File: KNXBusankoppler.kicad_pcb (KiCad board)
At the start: 2 copper layers, 42.2 x 37.3 mm, 6 parts, among them J1 Conn_01x10_Male, J2 Conn_01x04_Male, U1 ProMicro

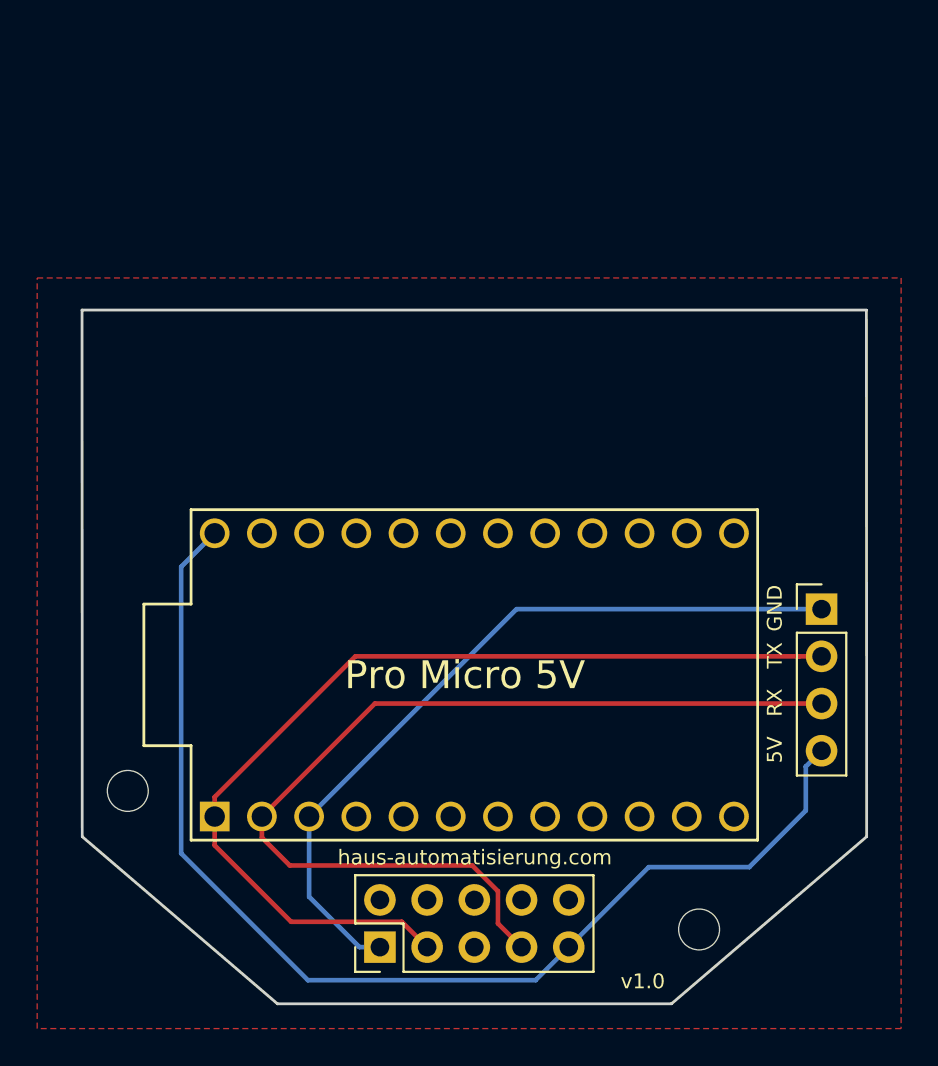
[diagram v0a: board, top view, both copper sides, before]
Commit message: CO2-Sensor 1.0
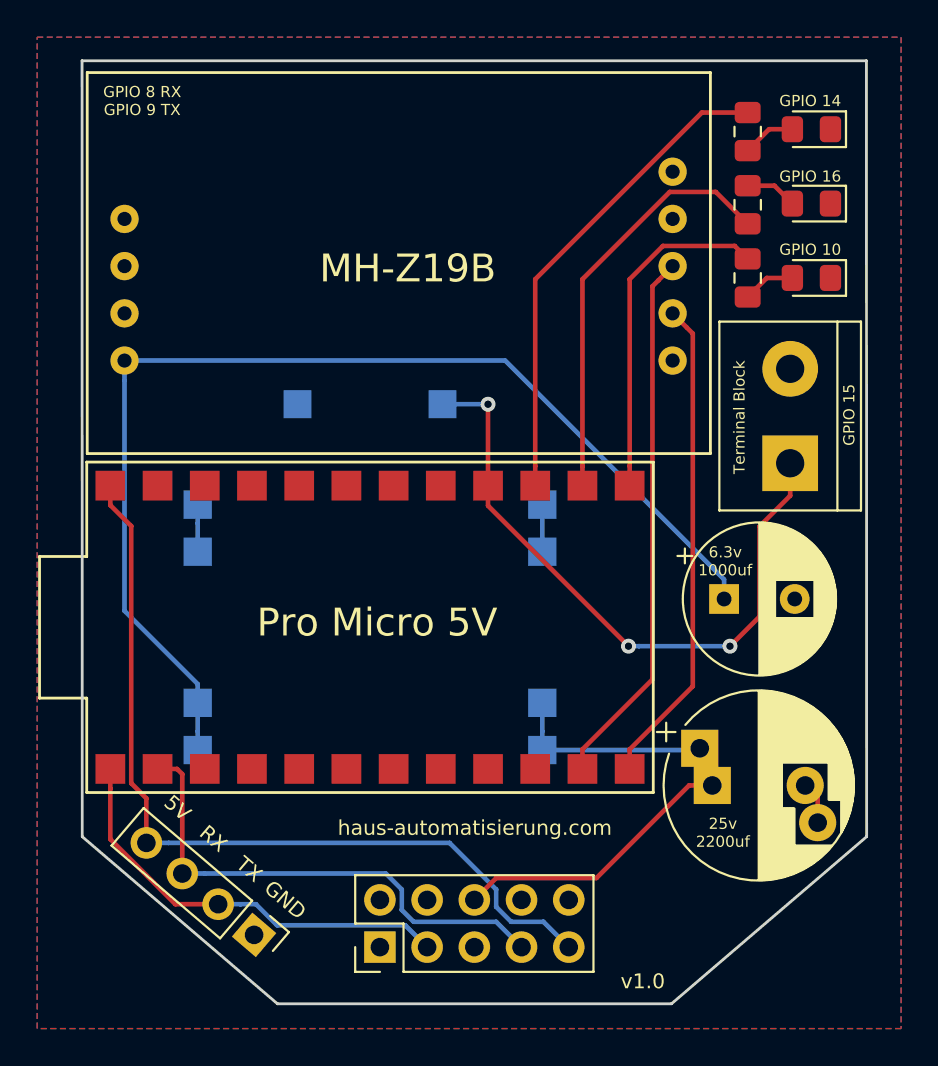
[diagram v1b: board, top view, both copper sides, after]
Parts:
- removed the REF** at (123.2, 102.8)
- removed the REF** at (154.0, 110.2)
- added C1: 25v 2200uf, Capacitor_THT:CP_Radial_D10.0mm_P5.00mm_P7.50mm, F.Cu at (154.7, 102.5)
- added C2: 6.3v 1000uf, Capacitor_THT:CP_Radial_D8.0mm_P3.80mm, F.Cu at (155.3, 92.5)
- added D1: LED, LED_SMD:LED_0805_2012Metric_Pad1.15x1.40mm_HandSolder, F.Cu at (160.0, 67.2)
- added D2: LED, LED_SMD:LED_0805_2012Metric_Pad1.15x1.40mm_HandSolder, F.Cu at (160.0, 71.2)
- added D3: LED, LED_SMD:LED_0805_2012Metric_Pad1.15x1.40mm_HandSolder, F.Cu at (160.0, 75.2)
- added J3: Screw_Terminal_01x02, TerminalBlock:TerminalBlock_bornier-2_P5.08mm, F.Cu at (158.9, 85.2)
- added R1: R, Resistor_SMD:R_0805_2012Metric_Pad1.15x1.40mm_HandSolder, F.Cu at (156.6, 67.3)
- added R2: R, Resistor_SMD:R_0805_2012Metric_Pad1.15x1.40mm_HandSolder, F.Cu at (156.6, 71.2)
- added R3: R, Resistor_SMD:R_0805_2012Metric_Pad1.15x1.40mm_HandSolder, F.Cu at (156.6, 75.2)
- added REF**: WEEE-Logo_4.2x6mm_SilkScreen, Symbol:WEEE-Logo_4.2x6mm_SilkScreen, B.Cu at (160.0, 67.5)
- added SW1: SW_Push, Button_Switch_SMD:SW_SPST_CK_RS282G05A3, B.Cu at (136.3, 82.0)
- added U2: MH_Z19B, libs:MH-Z19B, F.Cu at (123.1, 79.6)
- added U3: MP1584, libs:MP1584_buck_module_SMD, B.Cu at (136.3, 94.0)
- U1: footprint libs:ProMicro -> libs:ProMicroSMD
- moved J2 35.2 mm to (130.0, 110.5), turned to 229.5 degrees
- moved G*** 26.1 mm to (138.0, 70.7)
- moved U1 6.17 mm to (136.3, 94.0)
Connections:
- J1 pad 6: Net-(J1-Pad6) -> /20V
- U1 pad 23: Net-(U1-Pad23) -> GND
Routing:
- net Net-(C2-Pad1): track 0.00 -> 60.8 mm
- net Net-(J3-Pad1): track 0.00 -> 35.2 mm, vias 0 -> 3
- net GND: track 41.4 -> 8.29 mm
- net Net-(U1-Pad11): track 0.00 -> 29.1 mm
- net /TX: track 52.1 -> 23.2 mm
- net /20V: track 0.00 -> 28.7 mm
- net Net-(U1-Pad12): track 0.00 -> 26.4 mm
- net Net-(R1-Pad2): track 0.00 -> 26.3 mm
- net /RX: track 51.2 -> 27.3 mm
- net Net-(R2-Pad2): track 0.00 -> 22.7 mm
- net Net-(R3-Pad2): track 0.00 -> 18.5 mm
- net /5V: track 61.8 -> 45.6 mm
- net Net-(D1-Pad2): track 0.00 -> 2.88 mm
- net Net-(D3-Pad2): track 0.00 -> 2.83 mm
- net Net-(D2-Pad2): track 0.00 -> 2.80 mm
- added copper zone on B.Cu, net GND
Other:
- board size 42.2 x 37.3 mm -> 42.2 x 50.7 mm
- board text added: "25v 2200uf"
- board text added: "6.3v 1000uf"
- board text added: "CO2-Sensor"
- board text added: "GPIO 10"
- board text added: "GPIO 14"
- board text added: "GPIO 15"
- board text added: "GPIO 16"
- board text added: "GPIO 8 RX GPIO 9 TX"
- board text added: "MH-Z19B"
- board text added: "Terminal Block"
- board text added: "Test"
